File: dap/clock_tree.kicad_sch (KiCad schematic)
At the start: 4 parts, among them U3 AD9515, U4 ADF4351, U5 SN74AUC74RGYR, U6 SN74AUC74RGYR

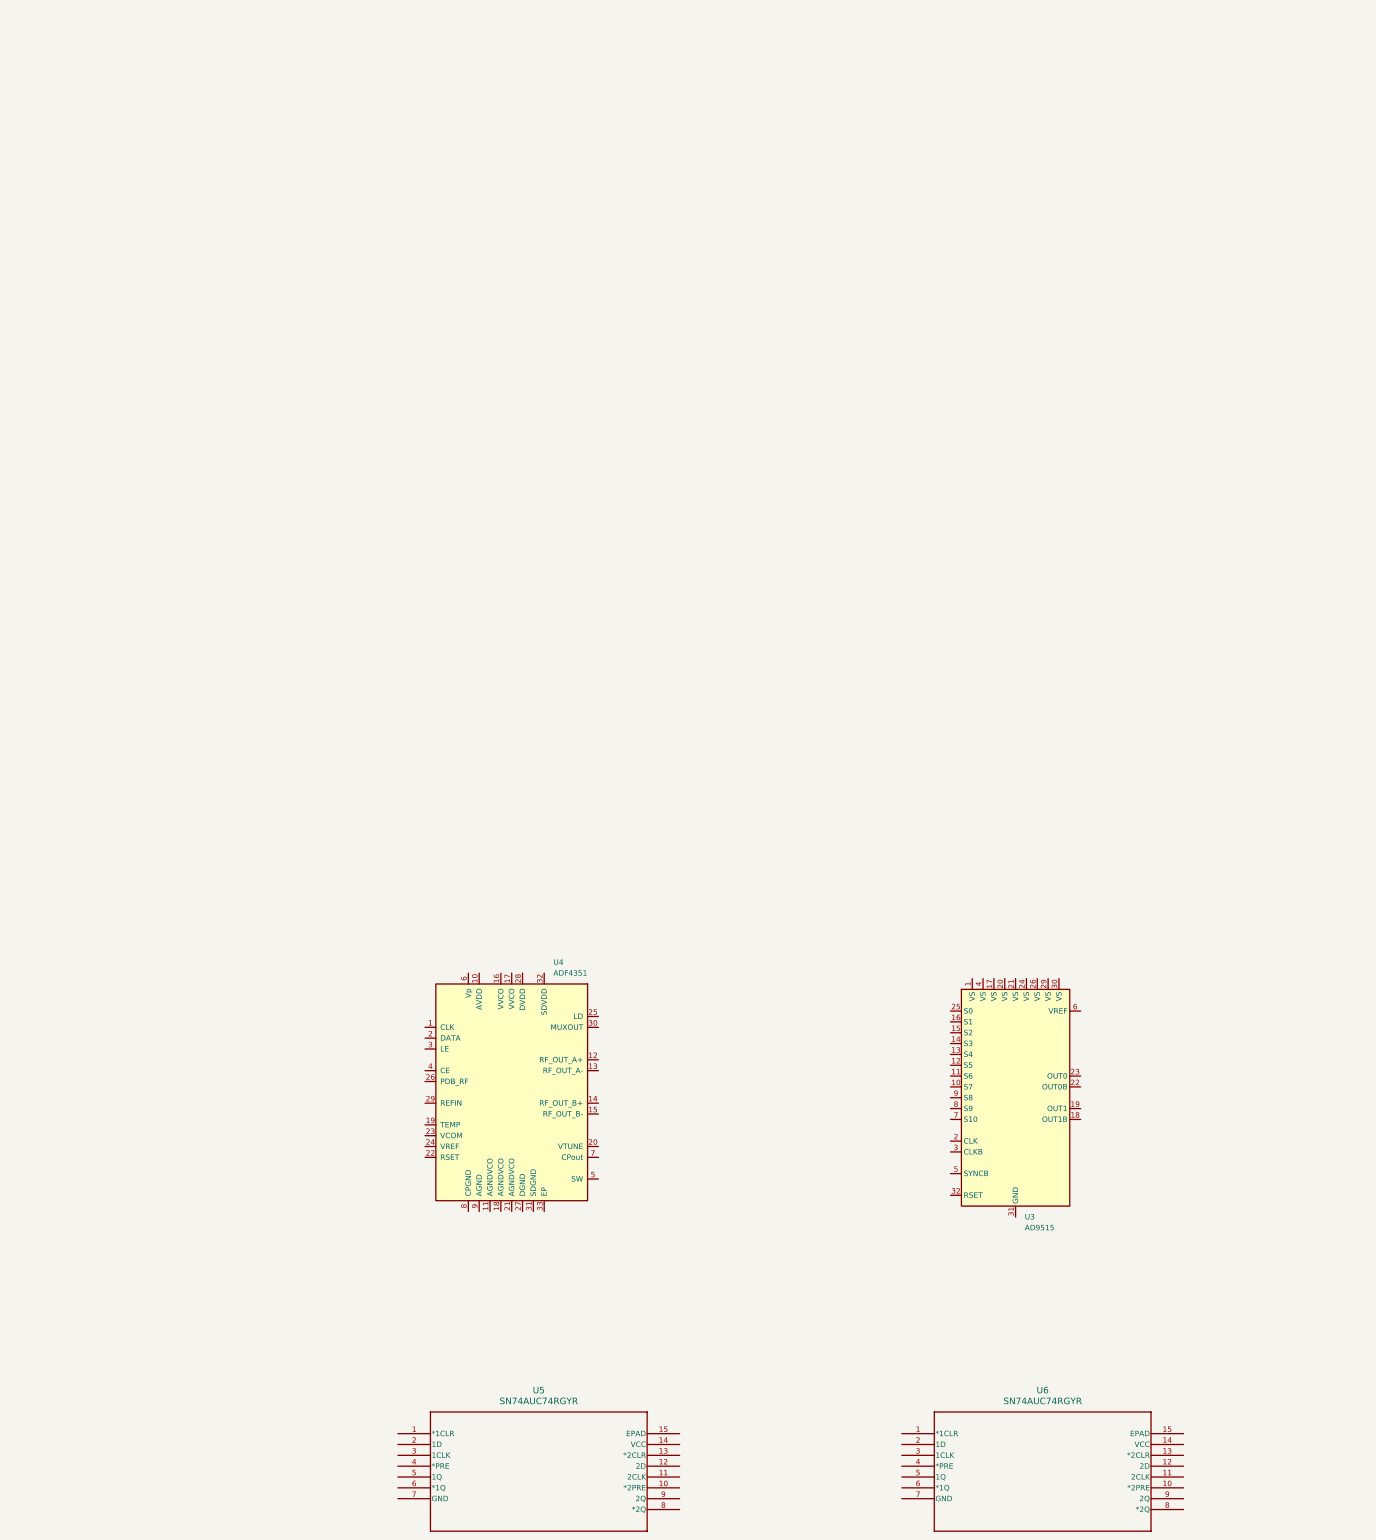
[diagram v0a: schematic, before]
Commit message: general setup
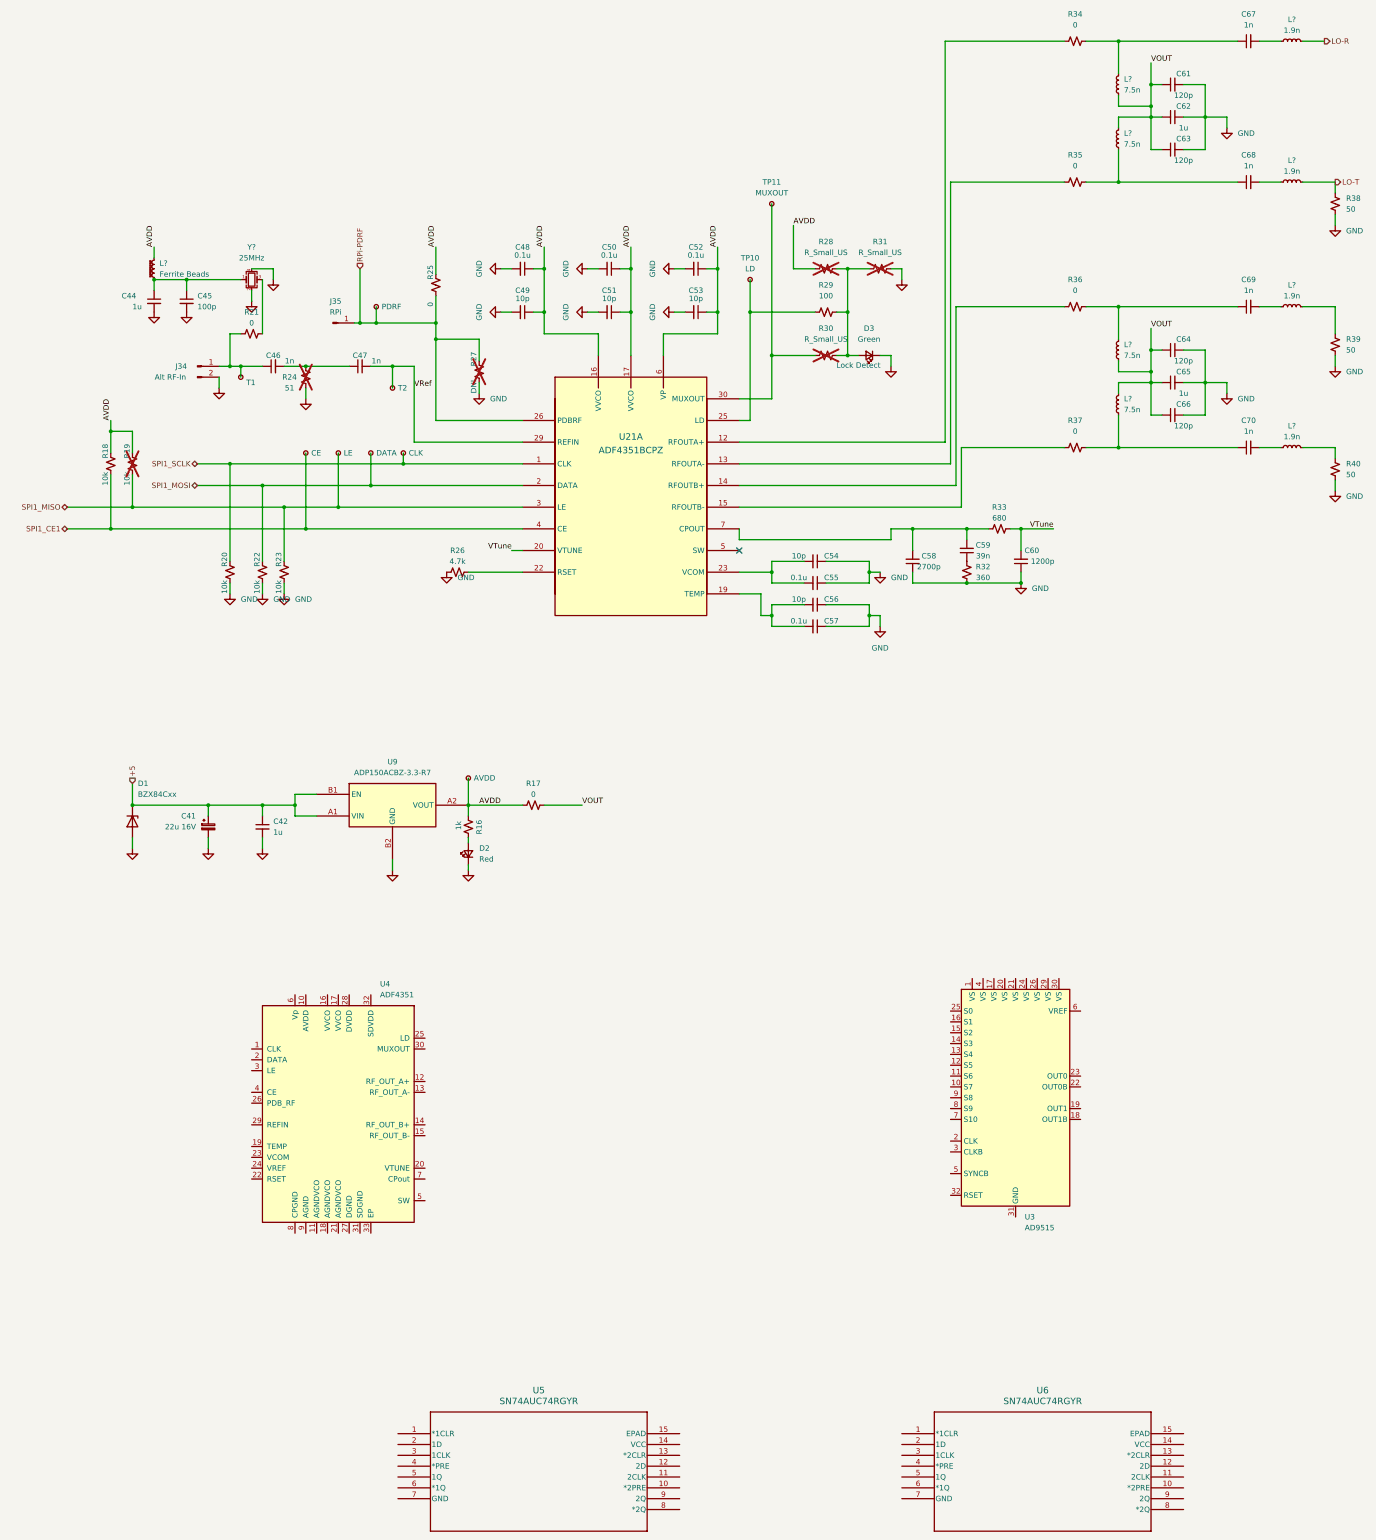
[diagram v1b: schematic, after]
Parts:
- added C41: 22u 16V, symbol Device:C_Polarized_Small
- added C42, C44, C62, C65: 1u, symbol Device:C_Small
- added C45: 100p, symbol Device:C_Small
- added C46, C47, C67, C68, C69, C70: 1n, symbol Device:C_Small
- added C48, C50, C52, C55, C57: 0.1u, symbol Device:C_Small
- added C49, C51, C53, C54, C56: 10p, symbol Device:C_Small
- added C58: 2700p, symbol Device:C_Small
- added C59: 39n, symbol Device:C_Small
- added C60: 1200p, symbol Device:C_Small
- added C61, C63, C64, C66: 120p, symbol Device:C_Small
- added D1: BZX84Cxx, Package_TO_SOT_SMD:SOT-23, symbol Diode:BZX84Cxx
- added D2: Red, symbol Device:LED_Small
- added D3: Green, symbol Device:LED_Small
- added J34: Alt RF-In, symbol Connector:Conn_01x02_Pin
- added J35: RPi, symbol Connector:Conn_01x01_Pin
- added L? (x4): 1.9n, symbol Device:L_Small
- added L?: Ferrite Beads, symbol Device:L_Ferrite_Small
- added L? (x4): 7.5n, symbol Device:L_Small
- added R16: 1k, symbol Device:R_Small_US
- added R17, R21, R25, R34, R35, R36, R37: 0, symbol Device:R_Small_US
- added R18, R19, R20, R22, R23: 10k, symbol Device:R_Small_US
- added R24: 51, symbol Device:R_Small_US
- added R26: 4.7k, symbol Device:R_Small_US
- added R27: DNI, symbol Device:R_Small_US
- added R28, R30, R31: R_Small_US, symbol Device:R_Small_US
- added R29: 100, symbol Device:R_Small_US
- added R32: 360, symbol Device:R_Small_US
- added R33: 680, symbol Device:R_Small_US
- added R38, R39, R40: 50, symbol Device:R_Small_US
- added TP1: AVDD, symbol Connector:TestPoint_Small
- added TP10: LD, symbol Connector:TestPoint_Small
- added TP11: MUXOUT, symbol Connector:TestPoint_Small
- added TP3: T1, symbol Connector:TestPoint_Small
- added TP4: CE, symbol Connector:TestPoint_Small
- added TP5: LE, symbol Connector:TestPoint_Small
- added TP6: DATA, symbol Connector:TestPoint_Small
- added TP7: PDRF, symbol Connector:TestPoint_Small
- added TP8: T2, symbol Connector:TestPoint_Small
- added TP9: CLK, symbol Connector:TestPoint_Small
- added U21: ADF4351BCPZ, hf-transceiver:CP-32-7_ADI, symbol hf-transceiver:ADF4351BCPZ
- added U9: ADP150ACBZ-3.3-R7, hf-transceiver:CB_4_3_ADI, symbol hf-transceiver:ADP150ACBZ-3.3-R7
- added Y?: 25MHz, symbol Device:Crystal_GND24_Small
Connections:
- new net: C56.2, C57.2, U21.19 (TEMP)
- new net: C54.2, C55.2, U21.23 (VCOM)
- new net: C44.1, C45.1, L?.1, Y?.1
- new net: D3.2 (A), R28.2, R29.2, R30.2, R31.1
- new net: C69.1, L?.2, R36.2
- new net: C69.2, L?.1
- new net: R34.1, U21.12 (RFOUTA+)
- new net: R35.1, U21.13 (RFOUTA-)
- new net: R36.1, U21.14 (RFOUTB+)
- new net: R37.1, U21.15 (RFOUTB-)
- new net: R26.2, U21.22 (RSET)
- new net: R29.1, TP10.1, U21.25 (LD)
- new net: R30.1, TP11.1, U21.30 (MUXOUT)
- new net: C58.2, C59.2, R33.1, U21.7 (CPOUT)
- new net: C70.1, L?.1, R37.2
- new net: C46.2, C47.1, R24.2
- new net: L?.2, R39.1
- new net: C46.1, J34.1 (Pin_1), R21.2, TP3.1
- new net: C59.1, R32.2
- new net: R21.1, Y?.3
- new net: C68.1, L?.1, R35.2
- new net: C70.2, L?.1
- new net: L?.2, R40.1
- new net: D2.2 (A), R16.2
- new net: C68.2, L?.1
- new net: C67.1, L?.2, R34.2
- new net: C67.2, L?.1
- new net +5: C41.1, C42.1, D1.3 (K), U9.A1 (VIN), U9.B1 (EN)
- new net AVDD: C48.1, C49.1, C50.1, C51.1, C52.1, C53.1, L?.2, R16.1, R17.2, R18.1, R19.1, R25.1, R28.1, TP1.1, U21.16 (VVCO), U21.17 (VVCO), U21.6 (VP), U9.A2 (VOUT)
- new net GND: C41.2, C42.2, C44.2, C45.2, C48.2, C49.2, C50.2, C51.2, C52.2, C53.2, C54.1, C55.1, C56.1, C57.1, C58.1, C60.1, C61.2, C62.2, C63.2, C64.2, C65.2, C66.2, D1.1 (A), D2.1 (K), D3.1 (K), J34.2 (Pin_2), R20.2, R22.2, R23.2, R24.1, R26.1, R27.2, R31.2, R32.1, R38.2, R39.2, R40.2, U9.B2 (GND), Y?.2, Y?.4
- new net LO-R: L?.2
- new net LO-T: L?.2, R38.1
- new net RPi-PDRF: J35.1 (Pin_1), R25.2, R27.1, TP7.1, U21.26 (PDBRF)
- new net SPI1_CE1: R18.2, TP4.1, U21.4 (CE)
- new net SPI1_MISO: R19.2, R23.1, TP5.1, U21.3 (LE)
- new net SPI1_MOSI: R22.1, TP6.1, U21.2 (DATA)
- new net SPI1_SCLK: R20.1, TP9.1, U21.1 (CLK)
- new net VOUT: C61.1, C62.1, C63.1, C64.1, C65.1, C66.1, L?.1, L?.1, L?.2, L?.2, R17.1
- new net VRef: C47.2, TP8.1, U21.29 (REFIN)
- new net VTune: C60.2, R33.2, U21.20 (VTUNE)
- no-connect marks 0 -> 1
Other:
- note added: "Lock Detect"
- moved on the sheet: U4
